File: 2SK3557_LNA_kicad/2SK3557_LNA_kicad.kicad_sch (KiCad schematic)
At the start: 12 parts, among them Q1 BF862

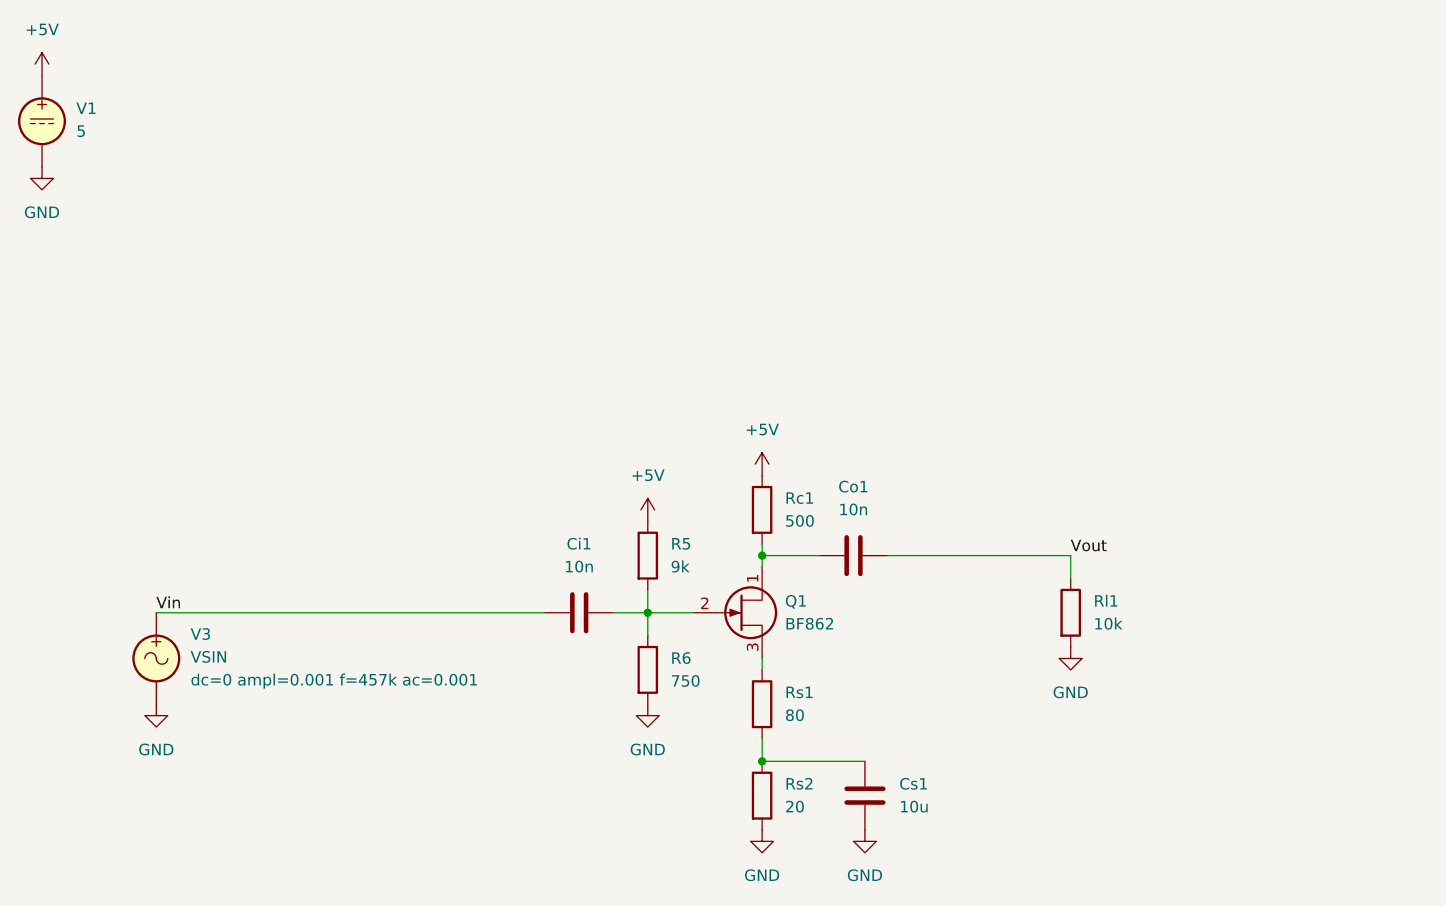
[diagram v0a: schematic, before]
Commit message: add all changes
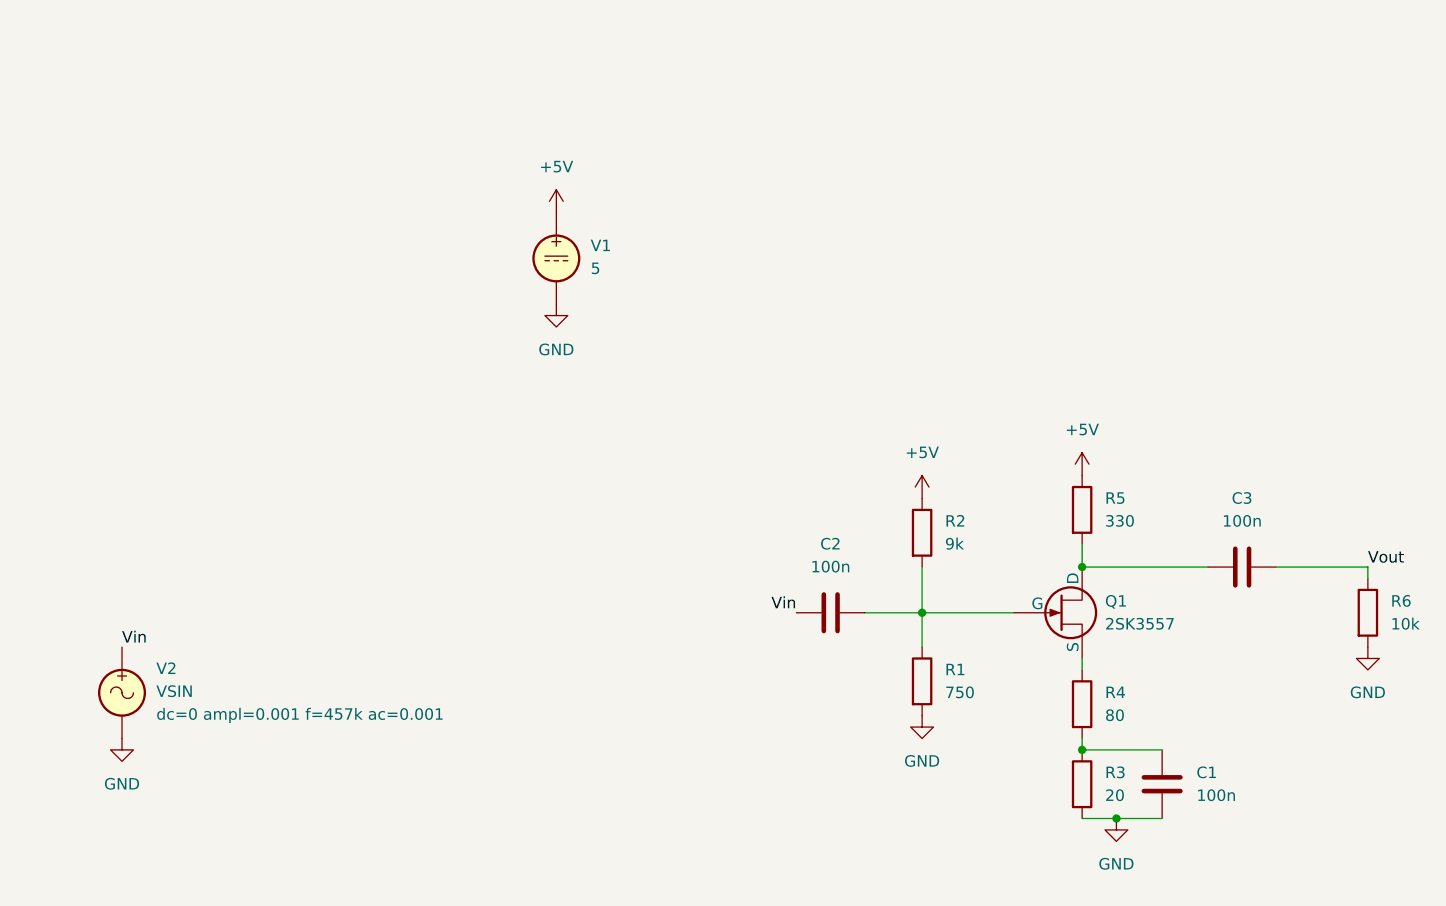
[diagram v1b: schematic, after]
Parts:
- removed Ci1, Co1: 10n, symbol Device:C
- removed Cs1: 10u, symbol Device:C
- removed Q1: BF862, Package_TO_SOT_THT:TO-92, symbol Transistor_FET:2N3819
- removed Rc1: 500, symbol Device:R
- removed Rl1: 10k, symbol Device:R
- removed Rs1: 80, symbol Device:R
- removed Rs2: 20, symbol Device:R
- removed V3: VSIN, symbol Simulation_SPICE:VSIN
- added C1, C2, C3: 100n, symbol Device:C
- added Q1: 2SK3557, symbol Simulation_SPICE:NJFET
- added R1: 750, symbol Device:R
- added R2: 9k, symbol Device:R
- added R3: 20, symbol Device:R
- added R4: 80, symbol Device:R
- added V2: VSIN, symbol Simulation_SPICE:VSIN
- R5: value 9k -> 330
- R6: value 750 -> 10k
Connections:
- net +5V: now also R2.1
- net GND: now also C1.2, R1.2, R3.2, V2.2
- net Vin: now also C2.1, V2.1
- net Vout: now also R6.1, C3.2
- net at R5.2: now also C3.1, Q1.1 (D); no longer R6.1
- new net: C1.1, R3.1, R4.2
- new net: C2.2, Q1.2 (G), R1.1, R2.2
- new net: Q1.3 (S), R4.1
